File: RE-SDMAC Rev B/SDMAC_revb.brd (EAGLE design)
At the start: 100 x 80 mm, 13 parts, among them IC1 SUPER_DMAC_THT, U1 74ALVC164245DGGRE4DGG48-M, U3 74ALVC164245DGGRE4DGG48-M, U4 74ALVC164245DGGRE4DGG48-M, U5 74ALVC164245DGGRE4DGG48-M

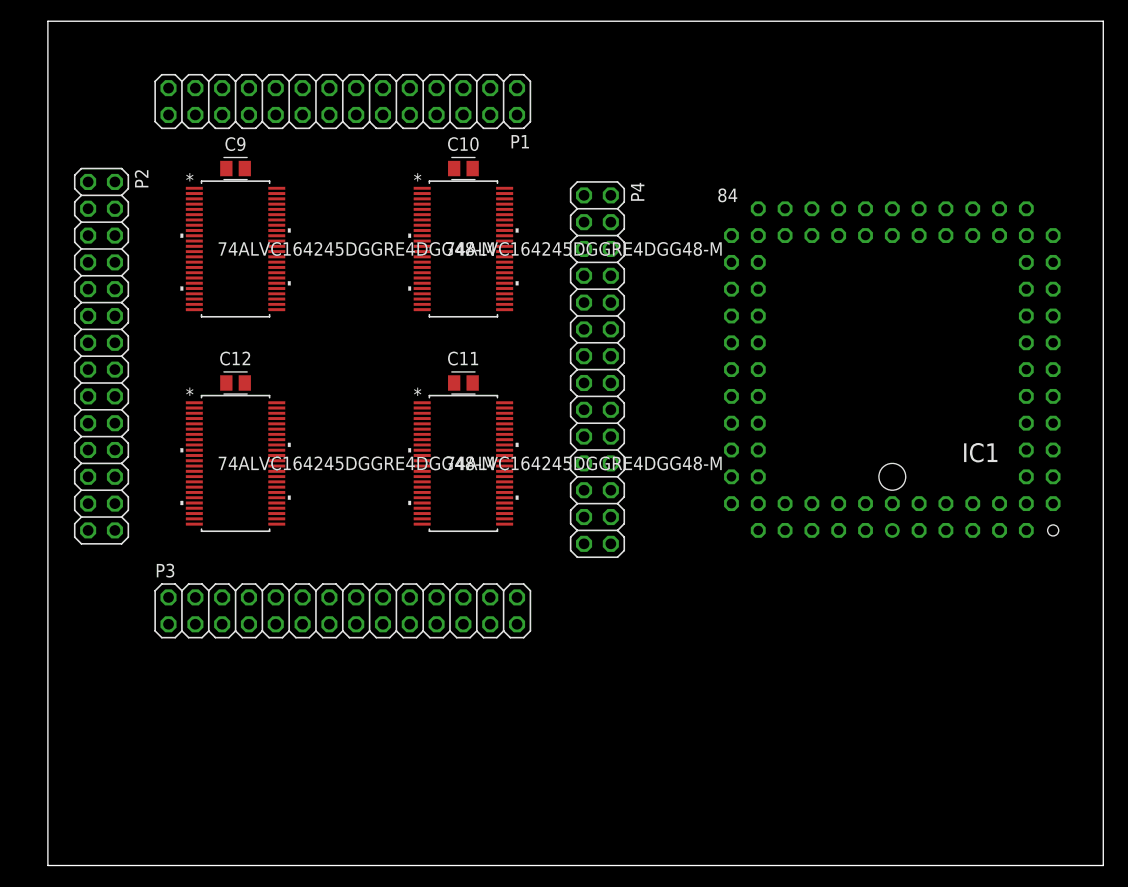
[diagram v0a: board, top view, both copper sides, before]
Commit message: more updates
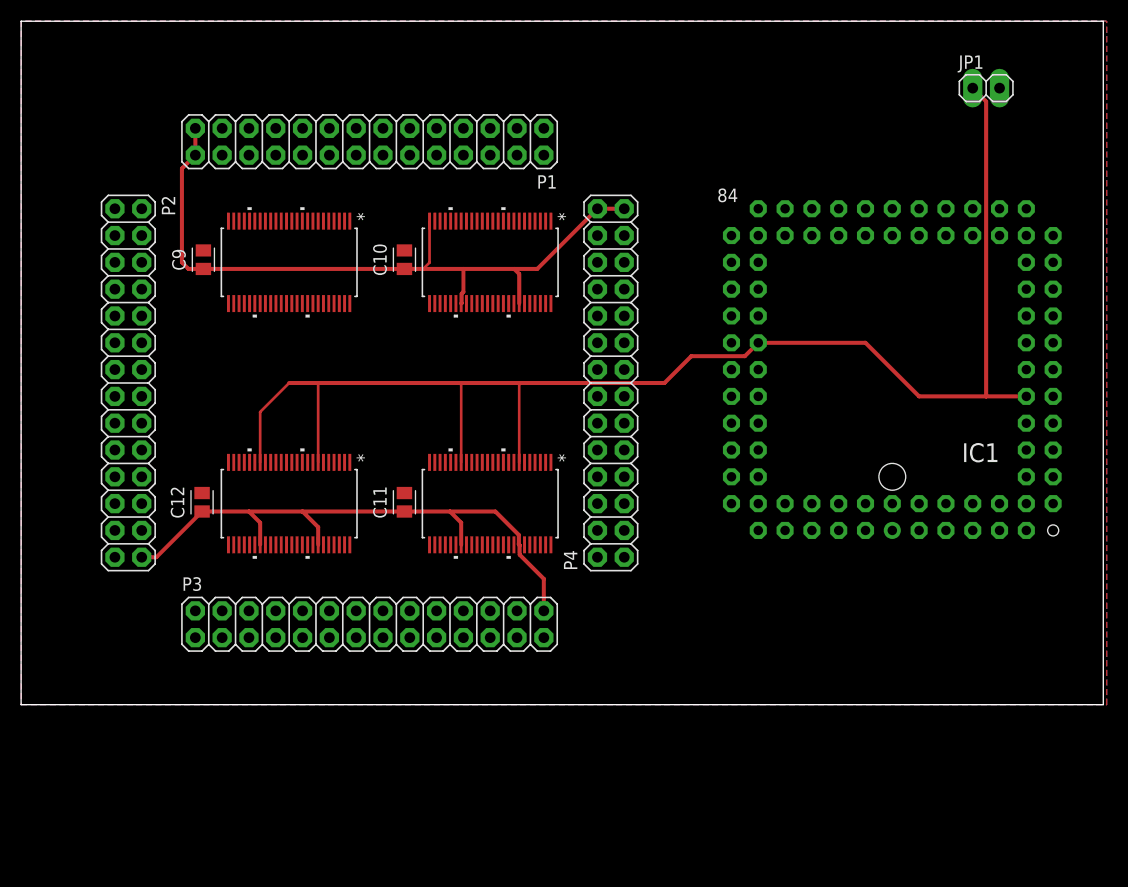
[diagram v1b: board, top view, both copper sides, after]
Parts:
- added JP1: (no value), pinhead:1X02
- moved U5 34.1 mm to (41.9, 34.3), turned to 270 degrees
- moved U4 30.7 mm to (41.9, 57.1), turned to 270 degrees
- moved U1 29.2 mm to (22.9, 34.3), turned to 270 degrees
- moved U3 25.2 mm to (22.9, 57.1), turned to 270 degrees
- moved C11 12.6 mm to (33.8, 34.4), turned to 90 degrees
- moved C12 11.7 mm to (14.6, 34.4), turned to 90 degrees
- moved C10 10.3 mm to (33.8, 57.4), turned to 90 degrees
- moved C9 9.16 mm to (14.7, 57.4), turned to 90 degrees
- moved P1 4.58 mm to (30.5, 68.6)
- moved P2 3.59 mm to (7.62, 45.7)
- moved P3 2.84 mm to (30.5, 22.9)
- moved P4 1.80 mm to (53.3, 45.7), turned to 90 degrees
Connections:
- removed net P1-1: U4.30
- new net P1_HDR1: P1.1, U4.30
- new net P1_HDR10: P1.10, U5.43
- new net P1_HDR11: P1.11, U5.41
- new net P1_HDR12: P1.12, U4.48
- new net P1_HDR13: P1.13
- new net P1_HDR14: P1.14
- new net P1_HDR15: P1.15, U4.36
- new net P1_HDR16: P1.16, U4.33
- new net P1_HDR17: P1.17
- new net P1_HDR18: P1.18, U4.27
- new net P1_HDR19: P1.19
- new net P1_HDR2: P1.2, U4.32
- new net P1_HDR20: P1.20
- new net P1_HDR22: P1.22, U3.46
- new net P1_HDR23: P1.23, U3.37
- new net P1_HDR24: P1.24, U3.40
- new net P1_HDR3: P1.3, U4.29
- new net P1_HDR4: P1.4, U4.35
- new net P1_HDR5: P1.5, U1.27
- new net P1_HDR6: P1.6
- new net P1_HDR7: P1.7, U4.44
- new net P1_HDR8: P1.8, U5.32
- new net P1_HDR9: P1.9, U4.38
- new net P2_HDR10: P2.10, U3.35
- new net P2_HDR11: P2.11, U3.32
- new net P2_HDR12: P2.12, U5.37
- new net P2_HDR13: P2.13, U5.35
- new net P2_HDR14: P2.14, U5.26
- new net P2_HDR15: P2.15
- new net P2_HDR16: P2.16, U3.41
- new net P2_HDR17: P2.17, U3.38
- new net P2_HDR18: P2.18, U3.36
- new net P2_HDR19: P2.19, U3.33
- new net P2_HDR20: P2.20, U3.30
- new net P2_HDR21: P2.21, U4.46
- new net P2_HDR22: P2.22, U3.29
- new net P2_HDR23: P2.23, U3.27
- new net P2_HDR24: P2.24, U3.26
- new net P2_HDR25: P2.25
- new net P2_HDR26: P2.26
- new net P2_HDR3: P2.3
- new net P2_HDR4: P2.4, U3.44
- new net P2_HDR5: P2.5, U3.43
- new net P2_HDR6: P2.6
- new net P2_HDR7: P2.7, U4.47
- new net P2_HDR8: P2.8
- new net P2_HDR9: P2.9
- new net P3_HDR10: P3.10, U1.38
- new net P3_HDR11: P3.11, U1.36
- new net P3_HDR12: P3.12, U1.33
- new net P3_HDR13: P3.13, U1.30
- new net P3_HDR14: P3.14
- new net P3_HDR15: P3.15, U3.47
- new net P3_HDR16: P3.16
- new net P3_HDR17: P3.17
- new net P3_HDR18: P3.18, U1.46
- new net P3_HDR19: P3.19, U1.43
- new net P3_HDR20: P3.20, U1.40
- new net P3_HDR21: P3.21, U1.37
- new net P3_HDR22: P3.22, U1.35
- new net P3_HDR23: P3.23, U1.32
- new net P3_HDR24: P3.24, U1.29
- new net P3_HDR25: P3.25
- new net P3_HDR3: P3.3, U4.26
- new net P3_HDR4: P3.4
- new net P3_HDR5: P3.5
- new net P3_HDR6: P3.6, U1.47
- new net P3_HDR7: P3.7, U1.44
- new net P3_HDR8: P3.8, U1.41
- new net P3_HDR9: P3.9, U1.26
- new net P4_HDR11: P4.11, U5.36
- new net P4_HDR12: P4.12
- new net P4_HDR13: P4.13, U5.46
- new net P4_HDR14: P4.14, U5.47
- new net P4_HDR15: P4.15, U4.37
- new net P4_HDR16: P4.16, U4.40
- new net P4_HDR17: P4.17
- new net P4_HDR18: P4.18
- new net P4_HDR21: P4.21, U5.44
- new net P4_HDR22: P4.22, U5.33
- new net P4_HDR23: P4.23, U5.38
- new net P4_HDR24: P4.24, U5.40
- new net P4_HDR3: P4.3
- new net P4_HDR4: P4.4, U4.43
- new net P4_HDR5: P4.5
- new net P4_HDR6: P4.6, U4.41
- new net P4_HDR7: P4.7
- net !CSS: no longer U4.48
- net !DATAOE: now also P1.21
- net GND: now also JP1.2, P1.25, P1.26, P2.1, P2.2, P2.27, P3.1, P3.2, P3.26, P3.27, P4.1, P4.10, P4.2, P4.25, P4.26, P4.8, P4.9, U5.27, U5.29, U5.30
- net VCC3.3: now also P1.27, P1.28, P2.28, P3.28, P4.27, P4.28
- net VCC5: now also JP1.1
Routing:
- net VCC5: track 0.00 -> 134.6 mm
- net VCC3.3: track 0.00 -> 127.0 mm
- added copper zone on layer 1, net GND
- added copper zone on layer 16, net GND
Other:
- board size 100 x 80 mm -> 102.5 x 64.8 mm
